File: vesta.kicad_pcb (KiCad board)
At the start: 2 copper layers, 39 parts, among them J1 Solar Panel, J2 Solar Panel, J4 Conn_02x07_Odd_Even, U2 BQ24074RGTR, U3 TPS63900DSKR, U4 BME688_C3664478, U5 RAK3172-T-8-SM-I

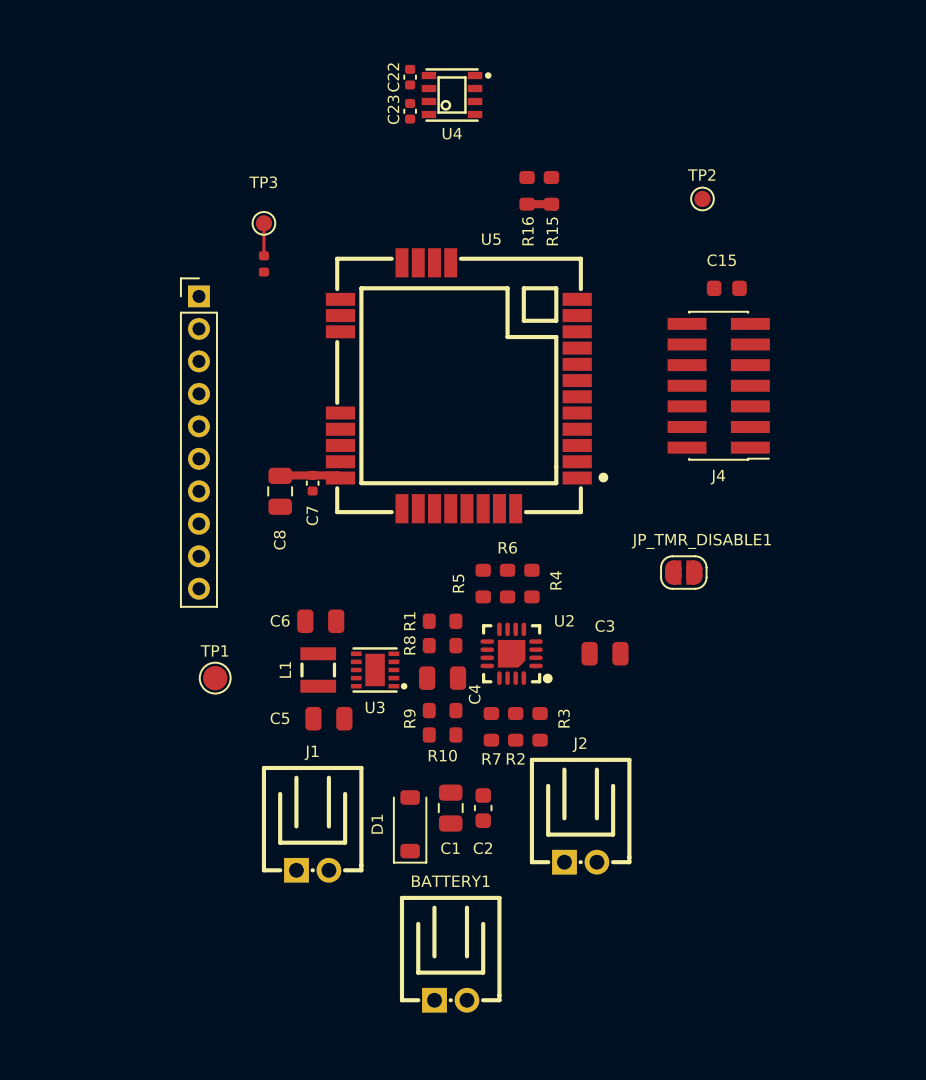
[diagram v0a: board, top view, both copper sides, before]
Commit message: feat: PCB design ready
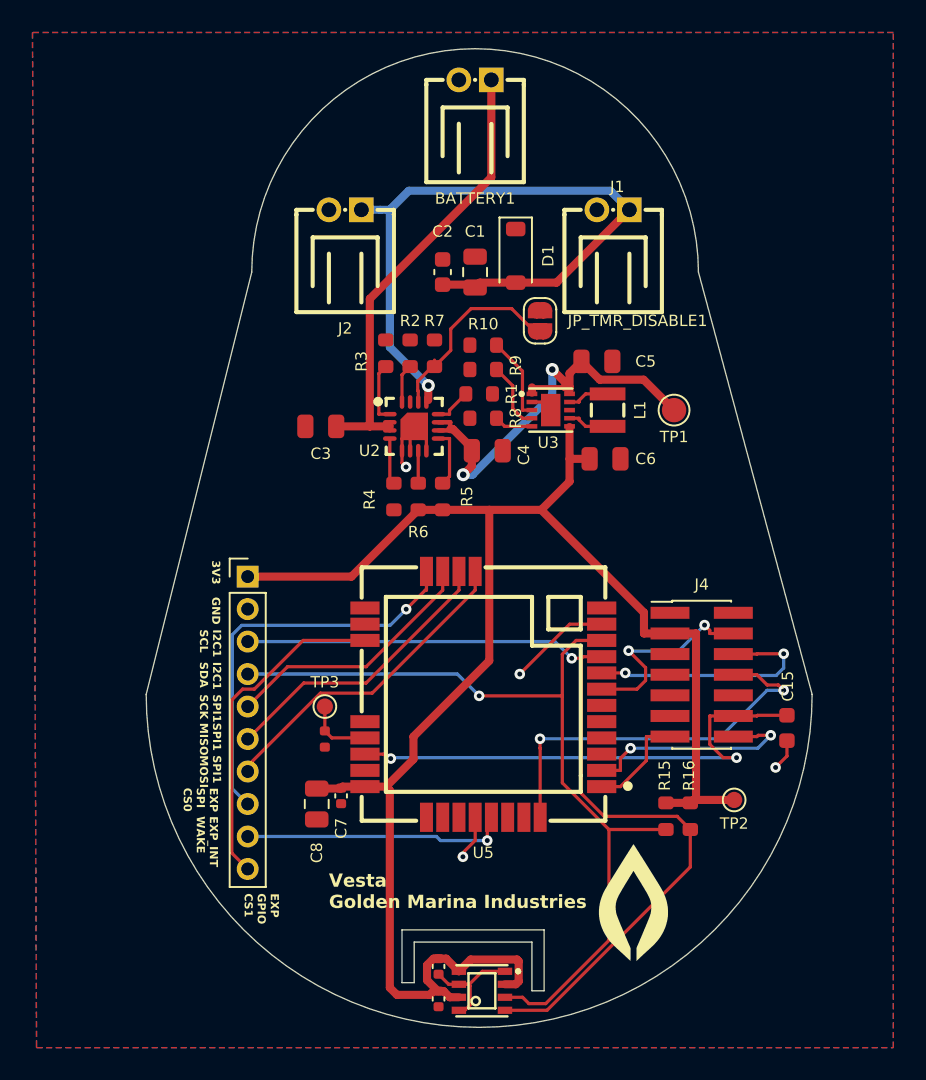
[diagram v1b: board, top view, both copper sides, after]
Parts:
- added G***: LOGO, Logo:logo, F.Cu at (54.3, 77.0)
- moved BATTERY1 56.7 mm to (44.5, 22.7), turned to 180 degrees
- moved U4 55.2 mm to (44.9, 78.8)
- moved C22 54.8 mm to (42.2, 77.2)
- moved C23 54.7 mm to (42.2, 79.2)
- moved J1 44.7 mm to (53.0, 30.7), turned to 180 degrees
- moved J2 42.7 mm to (36.5, 30.7), turned to 180 degrees
- moved R16 39.8 mm to (57.8, 68.0), turned to 90 degrees
- moved R15 39.1 mm to (56.2, 68.0), turned to 90 degrees
- moved TP2 37.1 mm to (60.5, 67.0), turned to 180 degrees
- moved D1 35.6 mm to (47.0, 33.5), turned to -90 degrees
- moved C2 33.1 mm to (42.5, 34.5), turned to -90 degrees
- moved C1 33.0 mm to (44.5, 34.5), turned to -90 degrees
- moved TP1 32.7 mm to (56.8, 43.0), turned to 180 degrees
- moved TP3 30.0 mm to (35.2, 61.2)
- moved R11 29.5 mm to (35.2, 63.2)
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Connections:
- U5 pad 2: unconnected-(U5-PA2/UART2_TX-Pad2) -> /UART_TX
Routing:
- net /3V3_SYS: track 5.55 -> 106.5 mm
- net /I2C1_SCL: track 0.00 -> 55.6 mm, vias 0 -> 1
- net /I2C1_SDA: track 0.00 -> 53.2 mm, vias 0 -> 1
- net /VIN_SOLAR: track 0.00 -> 43.9 mm, vias 0 -> 1
- net /NRST: track 0.00 -> 31.5 mm, vias 0 -> 2
- net /BAT_RAW: track 0.00 -> 28.2 mm
- net /SYS_RAW: track 0.00 -> 28.1 mm, vias 0 -> 2
- net GND: track 0.00 -> 26.2 mm, vias 0 -> 4
- net /EXP_SPI_CS0: track 0.00 -> 25.1 mm, vias 0 -> 1
- net /SWO: track 0.00 -> 24.6 mm, vias 0 -> 2
- net /EXP_GPIO_CS1: track 0.00 -> 20.5 mm
- net /SPI1_MOSI: track 0.00 -> 20.0 mm
- net /SPI1_MISO: track 0.00 -> 18.0 mm
- net /EXP_INT_WAKE: track 0.00 -> 16.4 mm, vias 0 -> 1
- net /SPI1_SCK: track 0.00 -> 16.1 mm
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- added copper zone on B.Cu, net GND
- added copper zone on F.Cu, net GND
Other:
- board outline added: 41 x 60.2 mm
- board text added: "()()()()() ()()()()()()() ()()()()()()()()() ()()()()()()()()() ()()()()()()()()()()() ()()()()()()()()()()() ()()()()()()()()()()()() ()()()()()()()()()()()()() ()()()()()()()()()()()()()() ()()()()()()()()()()()()()()() ()()()()()()()()()()()()()()()() ()()()()()()()()()()()()()()()()() ()()()()()()()()()()()()()()()()() ()()()()()()()()()()()()()()()()() ()()()()()()()()()()()()()()()()() ()()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"
- board text added: "3V3"
- board text added: "EXP GPIO CS1"
- board text added: "EXP SPI CS0"
- board text added: "EXP_INT WAKE"
- board text added: "GND"
- board text added: "I2C1 SCL"
- board text added: "I2C1 SDA"
- board text added: "SPI1 MISO"
- board text added: "SPI1 MOSI"
- board text added: "SPI1 SCK"
- board text added: "Vesta Golden Marina Industries"
- board text removed: "()()() ()()()()() ()()()()()()() ()()()()()()()() ()()()()()()()()()()() ()()()()()()()()()()() ()()()()()()()()()()()() ()()()()()()()()()()()()() ()()()()()()()()()()()()()() ()()()()()()()()()()()()()()() ()()()()()()()()()()()()()()()() ()()()()()()()()()()()()()()()()() ()()()()()()()()()()()()()()()()() ()()()()()()()()()()()()()()()()() ()()()()()()()()()()()()()()()()() ()()()()()()()()()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"
